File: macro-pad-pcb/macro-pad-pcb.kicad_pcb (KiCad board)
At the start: 2 copper layers, 46 parts, among them SW1 SW_Push, SW2 RotaryEncoder, U1 PRTR5V0U2X, U2 ATmega32U4-A, Y1 Crystal_GND24_Small

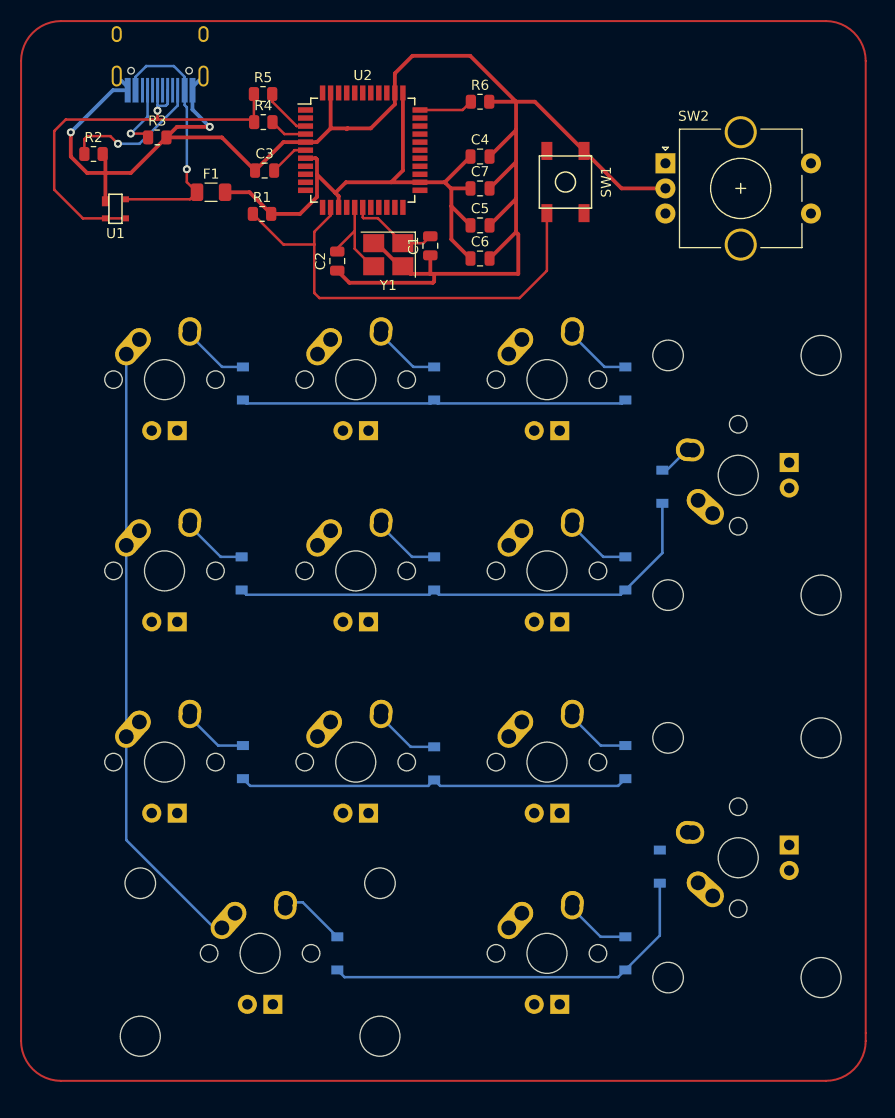
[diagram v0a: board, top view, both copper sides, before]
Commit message: Finished PCB
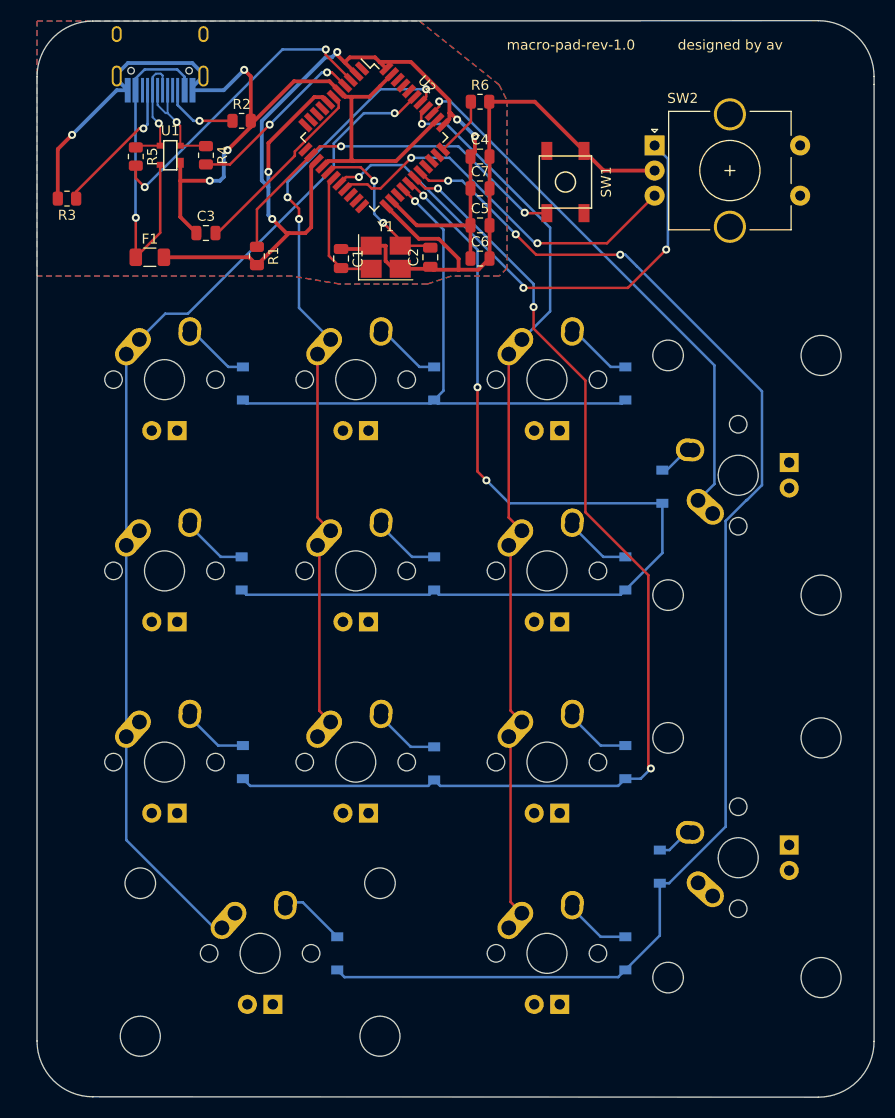
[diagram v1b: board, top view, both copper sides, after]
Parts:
- moved R2 15.1 mm to (180.7, 59.9)
- moved R5 14.1 mm to (170.2, 63.5), turned to -90 degrees
- moved R3 10.9 mm to (163.3, 67.7), turned to 180 degrees
- moved C2 9.28 mm to (199.5, 73.5)
- moved C1 8.98 mm to (190.6, 73.7), turned to -90 degrees
- moved F1 8.89 mm to (171.6, 73.5)
- moved C3 8.54 mm to (177.2, 71.1)
- moved U1 7.63 mm to (173.6, 63.4), turned to 180 degrees
- moved R4 6.60 mm to (177.2, 63.4), turned to -90 degrees
- moved R1 4.22 mm to (182.2, 73.4), turned to -90 degrees
- moved SW2 2.08 mm to (221.9, 62.4)
- moved U2 1.71 mm to (193.9, 61.6), turned to -45 degrees
- moved Y1 0.36 mm to (195.1, 73.5), turned to 0 degrees
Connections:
- R5 pad 1: D+ -> D-
- U1 pad 3: D+ -> D-
- U2 pad 18: unconnected-(U2-Pad18) -> EN2
- U2 pad 19: unconnected-(U2-Pad19) -> EN1
- U2 pad 26: unconnected-(U2-Pad26) -> ROW0
- U2 pad 27: unconnected-(U2-Pad27) -> ROW1
- U2 pad 28: unconnected-(U2-Pad28) -> ROW2
- U2 pad 29: unconnected-(U2-Pad29) -> ROW3
- U2 pad 36: unconnected-(U2-Pad36) -> COL3
- U2 pad 37: unconnected-(U2-Pad37) -> COL2
- U2 pad 38: unconnected-(U2-Pad38) -> COL1
- U2 pad 39: unconnected-(U2-Pad39) -> COL0
- USB1 pad 5: Net-(USB1-Pad5) -> D-
- USB1 pad 7: Net-(USB1-Pad5) -> D-
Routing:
- net ROW3: track 39.4 -> 136.2 mm, vias 0 -> 3
- net COL2: track 0.00 -> 87.4 mm, vias 0 -> 1
- net COL1: track 0.00 -> 76.8 mm, vias 0 -> 3
- net ROW2: track 39.2 -> 111.5 mm, vias 0 -> 3
- net COL3: track 0.00 -> 54.0 mm, vias 0 -> 1
- net ROW1: track 49.2 -> 100.5 mm, vias 0 -> 3
- net EN2: track 0.00 -> 51.1 mm, vias 0 -> 3
- net +5V: track 57.5 -> 102.5 mm, vias 0 -> 5
- net COL0: track 61.5 -> 100.4 mm, vias 0 -> 1
- net EN1: track 0.00 -> 37.9 mm, vias 0 -> 2
- net D+: track 42.9 -> 11.4 mm
- net Net-(R5-Pad2): track 5.08 -> 30.3 mm, vias 0 -> 2
- net ROW0: track 38.7 -> 61.7 mm, vias 0 -> 1
- net Net-(C3-Pad2): track 3.97 -> 19.0 mm
- net Net-(R4-Pad2): track 3.79 -> 18.2 mm, vias 0 -> 2
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- added copper zone on B.Cu, net GND
- added copper zone on F.Cu, net GND
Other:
- board outline added: 83.4 x 107.2 mm
- board text added: "designed by av"
- board text added: "macro-pad-rev-1.0"
